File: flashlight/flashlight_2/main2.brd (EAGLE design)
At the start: 20 x 20 mm, 10 parts

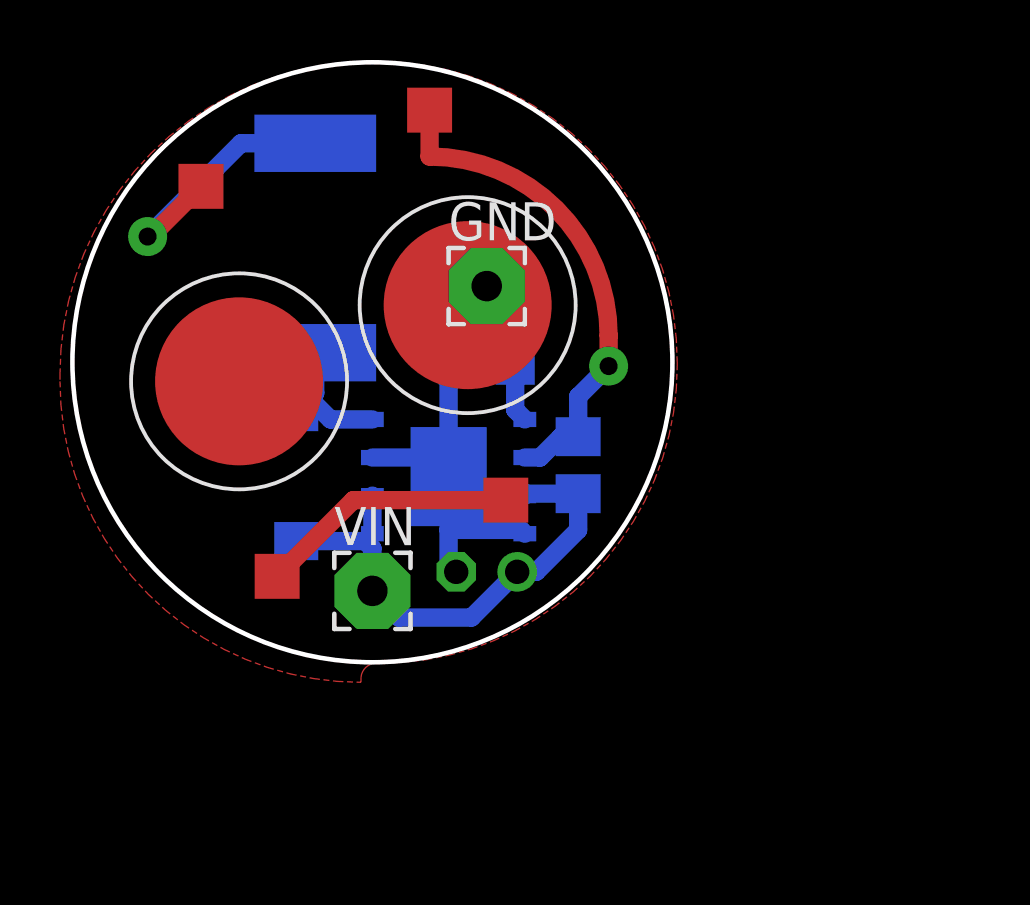
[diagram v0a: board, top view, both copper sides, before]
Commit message: updated project
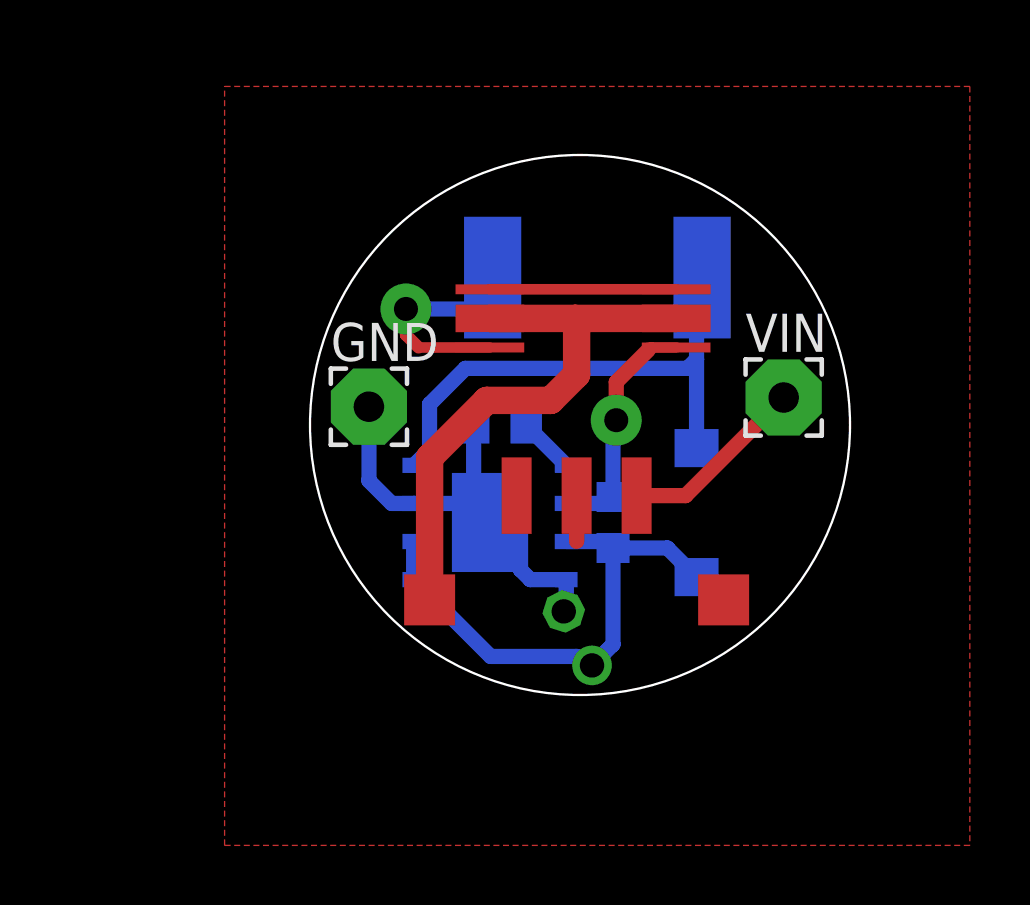
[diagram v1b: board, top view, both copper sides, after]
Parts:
- removed LED1, LED2: COBLED, 7_segment_lib:COBLED
- added U$2, U$4: XBDAWT_CREE_LED, 7_segment_lib:XBDAWT
- added U$5: SS312, 7_segment_lib:SS312
- C2: device rcl:C0805 -> rcl:C0603K
- R1: device resistor:R0805 -> resistor:R0603
- moved VIN 15.1 mm to (9.90, 1.37)
- moved D1 13.4 mm to (6.99, -2.47)
- moved U$3 9.46 mm to (3.69, 5.36), turned to 180 degrees
- moved GND 5.62 mm to (-3.93, 1.06)
- moved C1 3.76 mm to (3.04, -6.66), turned to 62.4 degrees
- moved R1 2.24 mm to (4.21, -2.80)
- moved C2 2.21 mm to (0.44, 0.37)
- moved U$1 2.06 mm to (0.11, -2.80)
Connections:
- new net N$8: U$5.P3, VIN.1
- net N$1: now also U$3.P$1, U$4.P$3; no longer LED1.P$2, LED2.P$1
- net N$3: now also U$5.P1; no longer VIN.1
- net N$5: now also U$2.P$2; no longer LED1.P$1
- net N$7: now also U$2.P$3, U$4.P$2; no longer LED2.P$2, U$3.P$1
- net PLANE: now also U$2.P$1, U$4.P$1, U$5.P4@1, U$5.P4@2; no longer LED1.P$3, LED2.P$3
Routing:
- net PLANE: track 0.00 -> 18.9 mm
- net N$6: track 4.62 -> 17.5 mm
- net N$5: track 15.8 -> 7.98 mm
- net N$8: track 0.00 -> 6.26 mm
- net N$7: track 9.35 -> 6.21 mm, vias 1 -> 0
- net N$3: track 17.1 -> 19.0 mm
- net N$2: track 15.6 -> 14.4 mm
- net N$1: track 8.67 -> 7.65 mm, vias 0 -> 1
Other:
- board size 20 x 20 mm -> 18 x 18 mm
